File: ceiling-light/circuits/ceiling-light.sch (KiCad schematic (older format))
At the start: 54 parts, among them J1 Screw_Terminal_01x03, J2 Screw_Terminal_01x02, P1 ESProg_Mating_Header, Q1 IRF840, Q2 IRF840, Q3 KSP44, SW1 SW_Push, SW2 SW_Push, U1 TMP36xS, U2 FL51xxMX, U3 AMS1117-3.3, U4 LTV-817, U5 DAC081C081CIMK, U6 ESP32-WROOM-32D

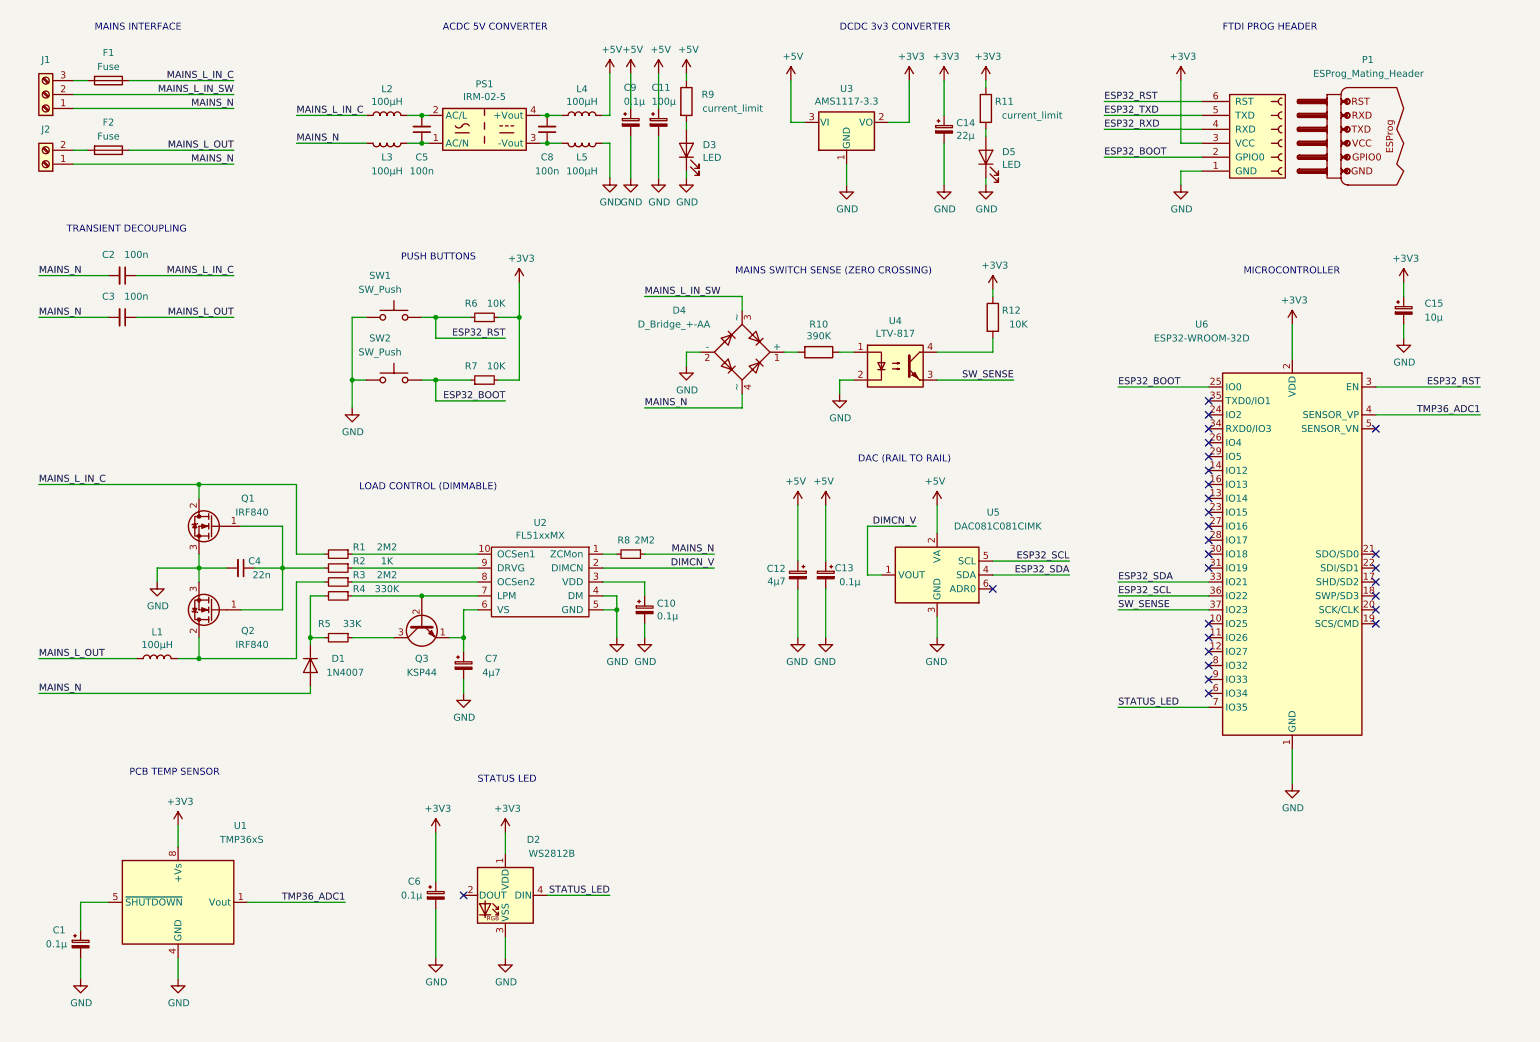
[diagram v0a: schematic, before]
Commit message: work on schematic
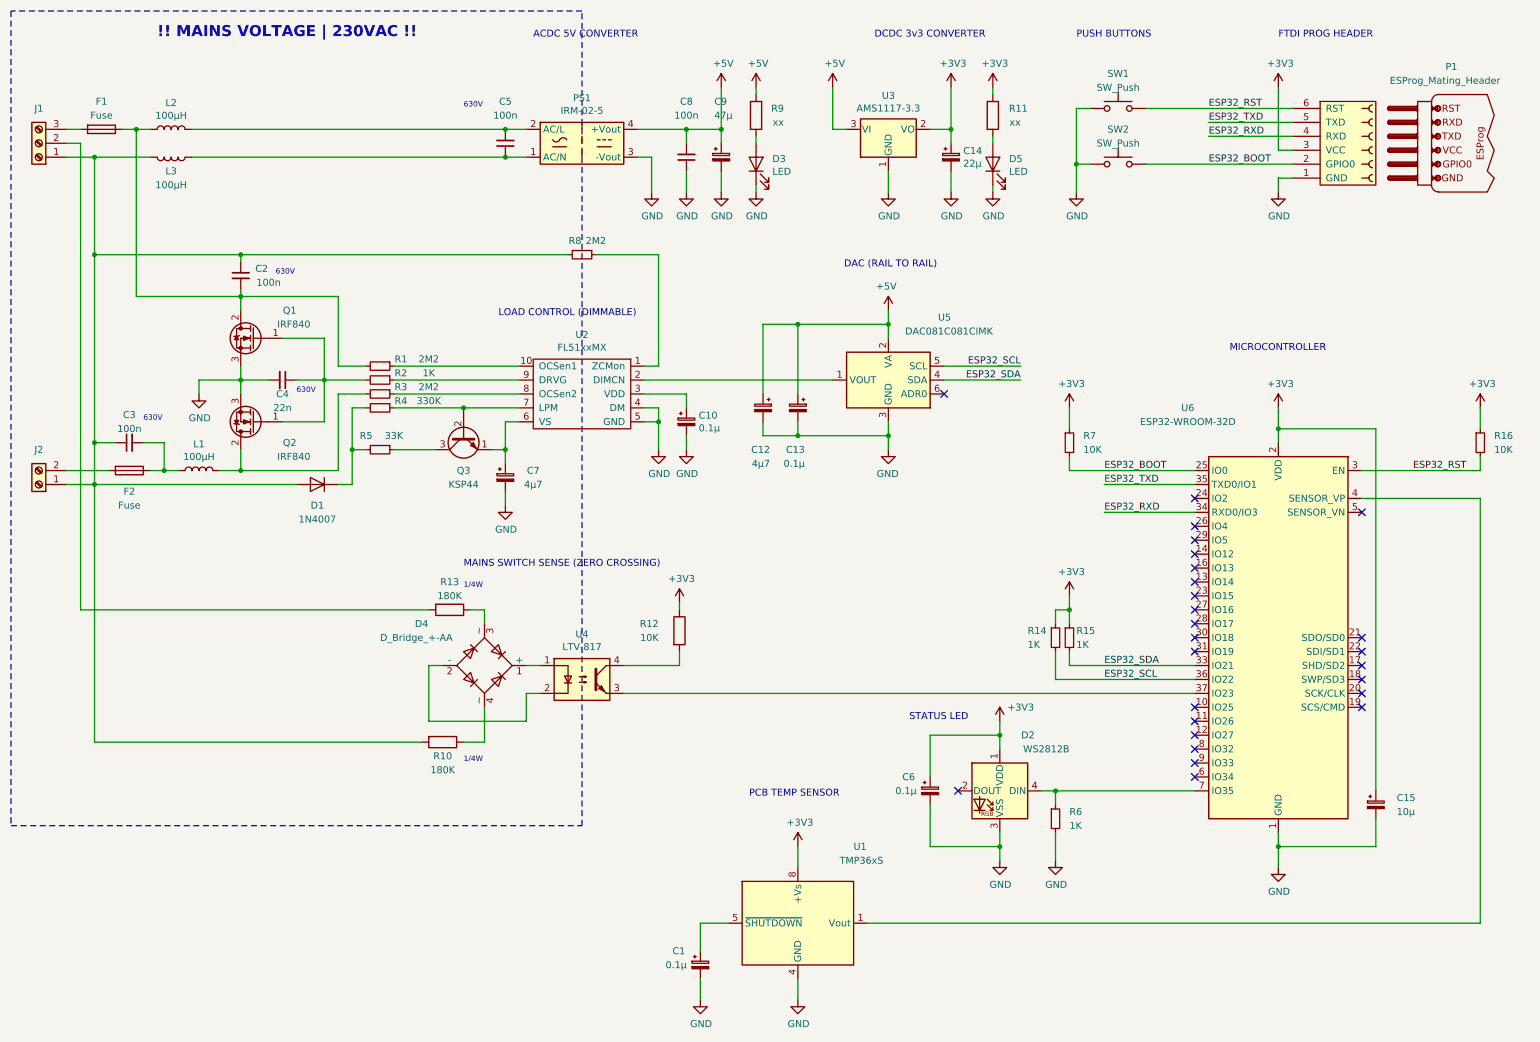
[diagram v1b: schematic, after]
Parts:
- removed C11: 100µ, Capacitor_SMD:C_1206_3216Metric_Pad1.42x1.75mm_HandSolder, symbol Device:CP_Small
- removed L4, L5: 100µH, Inductor_SMD:L_6.3x6.3_H3, symbol Device:L
- added R13: 180K, Resistor_SMD:R_1210_3225Metric_Pad1.42x2.65mm_HandSolder, symbol Device:R
- added R14, R15: 1K, Resistor_SMD:R_1210_3225Metric_Pad1.42x2.65mm_HandSolder, symbol Device:R_Small
- added R16: 10K, Resistor_SMD:R_1210_3225Metric_Pad1.42x2.65mm_HandSolder, symbol Device:R_Small
- C9: value 0.1µ -> 47µ
- R10: value 390K -> 180K
- R11, R9: value current_limit -> xx
- R6: value 10K -> 1K
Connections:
- net +3V3: now also R7.1, R14.1, R15.1, R16.1; no longer R6.2, R7.2
- net +5V: now also C8.2, PS1.4 (+Vout)
- net ESP32_BOOT: now also R7.2; no longer R7.1
- net ESP32_RST: now also R16.2; no longer R6.1
- net ESP32_RXD: now also U6.34 (RXD0/IO3)
- net ESP32_SCL: now also R14.2
- net ESP32_SDA: now also R15.2
- net ESP32_TXD: now also U6.35 (TXD0/IO1)
- net GND: now also C8.1, PS1.3 (-Vout), R6.2; no longer D4.2 (-), U4.2
- net at R8.2: now also C2.1, C3.1, D1.2 (A), J1.1 (Pin_1), J2.1 (Pin_1), L3.2, R10.2; no longer U2.1 (ZCMon)
- net at U4.1: now also D4.1 (+); no longer R10.1
- net DIMCN_V: no longer names the net of U2.2 (DIMCN), U5.1 (VOUT)
- net MAINS_L_IN_C: no longer names the net of F1.1, L2.1, Q1.2 (D), R1.2
- net MAINS_L_IN_C: now also C2.2; no longer C2.1
- net MAINS_L_IN_SW: no longer names the net of J1.2 (Pin_2)
- net MAINS_L_IN_SW: now also R13.2; no longer D4.3 (~~)
- net MAINS_L_OUT: no longer names the net of F2.1, L1.1
- net MAINS_L_OUT: now also C3.2; no longer C3.1
- removed net MAINS_N: C2.2, C3.2, D1.2 (A), D4.4 (~~), J1.1 (Pin_1), J2.1 (Pin_1), L3.2, R8.1
- net STATUS_LED: no longer names the net of D2.4 (DIN), U6.7 (IO35)
- net STATUS_LED: now also R6.1
- net SW_SENSE: no longer names the net of U4.3, U6.37 (IO23)
- net TMP36_ADC1: no longer names the net of U1.1 (Vout), U6.4 (SENSOR_VP)
- new net: R8.1, U2.1 (ZCMon)
- new net: D4.3 (~~), R13.1
- new net: D4.2 (-), U4.2
- new net: D4.4 (~~), R10.1
- no-connect marks 28 -> 26
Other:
- note added: "!! MAINS VOLTAGE | 230VAC !!"
- note added: "1/4W"
- note added: "630V"
- note removed: "MAINS INTERFACE"
- note removed: "TRANSIENT DECOUPLING"
- moved on the sheet: C1, C10, C12, C13, C14, C15, C2, C3, C4, C5, C6, C7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
